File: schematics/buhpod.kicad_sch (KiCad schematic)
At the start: 7 parts, among them J1 Micro SD Card Reader Module, SW1 PLAY_PAUSE, SW2 PREVIOUS, SW3 NEXT, SW4 VolumeControls

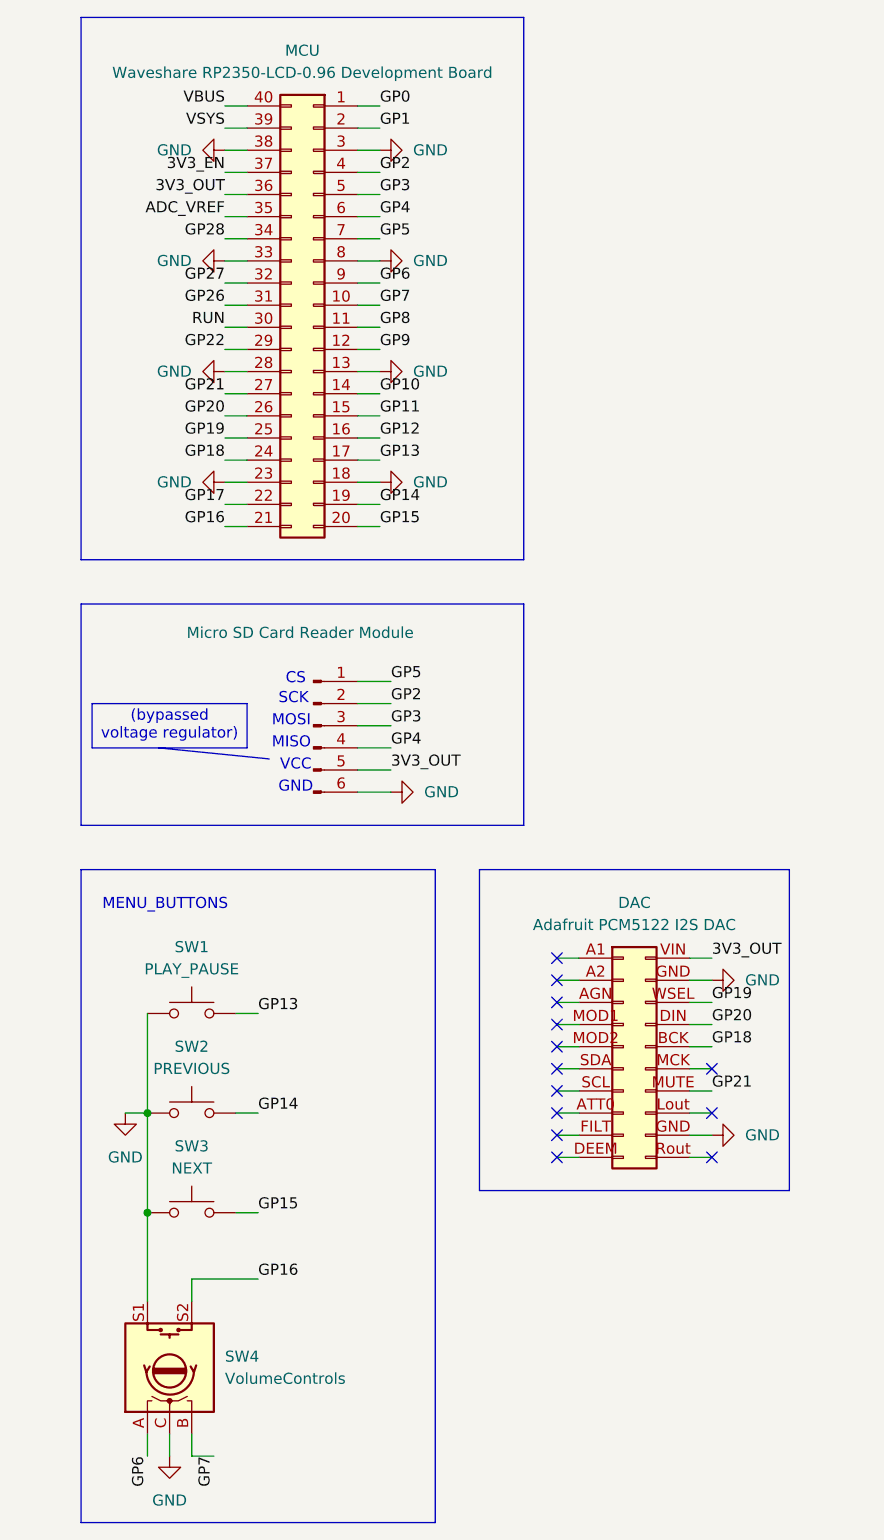
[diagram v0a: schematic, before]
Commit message: added misc btn
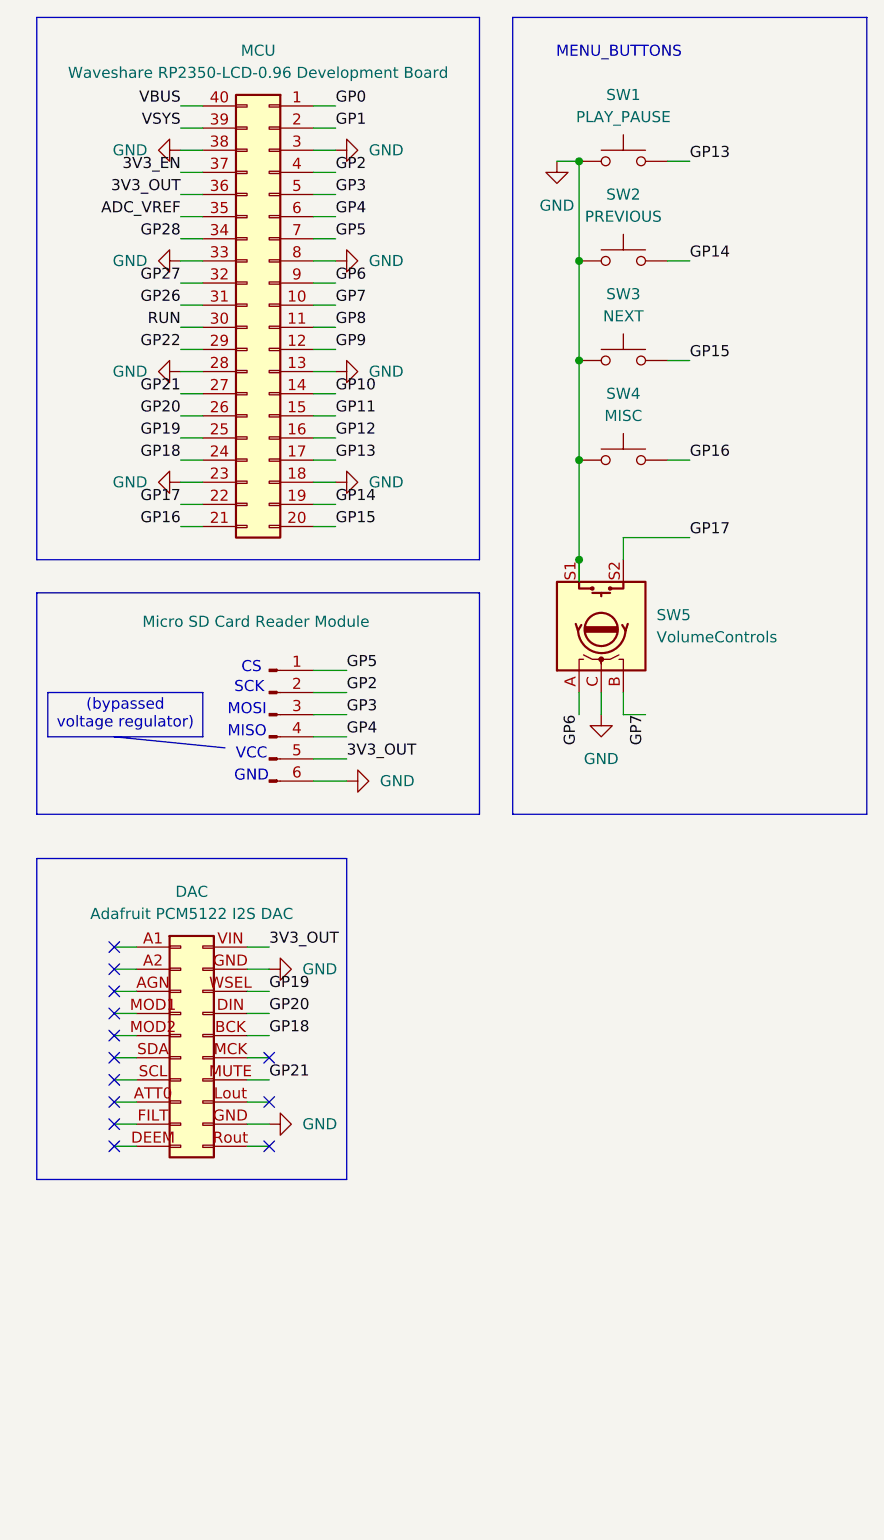
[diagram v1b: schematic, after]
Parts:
- added SW4: MISC, symbol Switch:SW_Push
- renumbered SW4 to SW5
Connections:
- net GND: now also SW4.1
- net GP16: now also SW4.2; no longer SW5.S2
- net GP17: now also SW5.S2
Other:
- moved on the sheet: DAC, MCU, SW1, SW2, SW3, SW5
